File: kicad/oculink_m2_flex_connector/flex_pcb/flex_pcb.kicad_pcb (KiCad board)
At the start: 2 copper layers, 42 x 20 mm, 3 parts, among them J1 Conn_02x01, J2 Conn_02x01

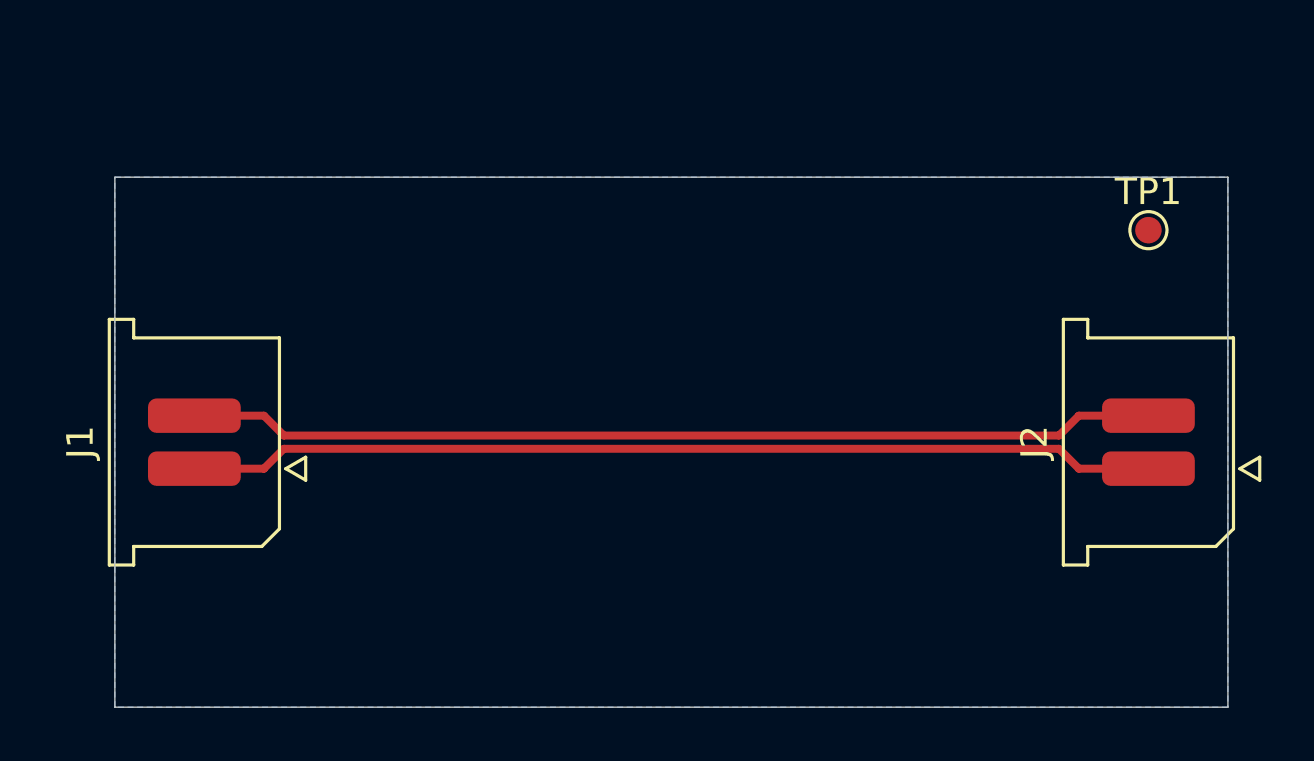
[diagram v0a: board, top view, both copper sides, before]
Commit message: Crude flex pcb layout
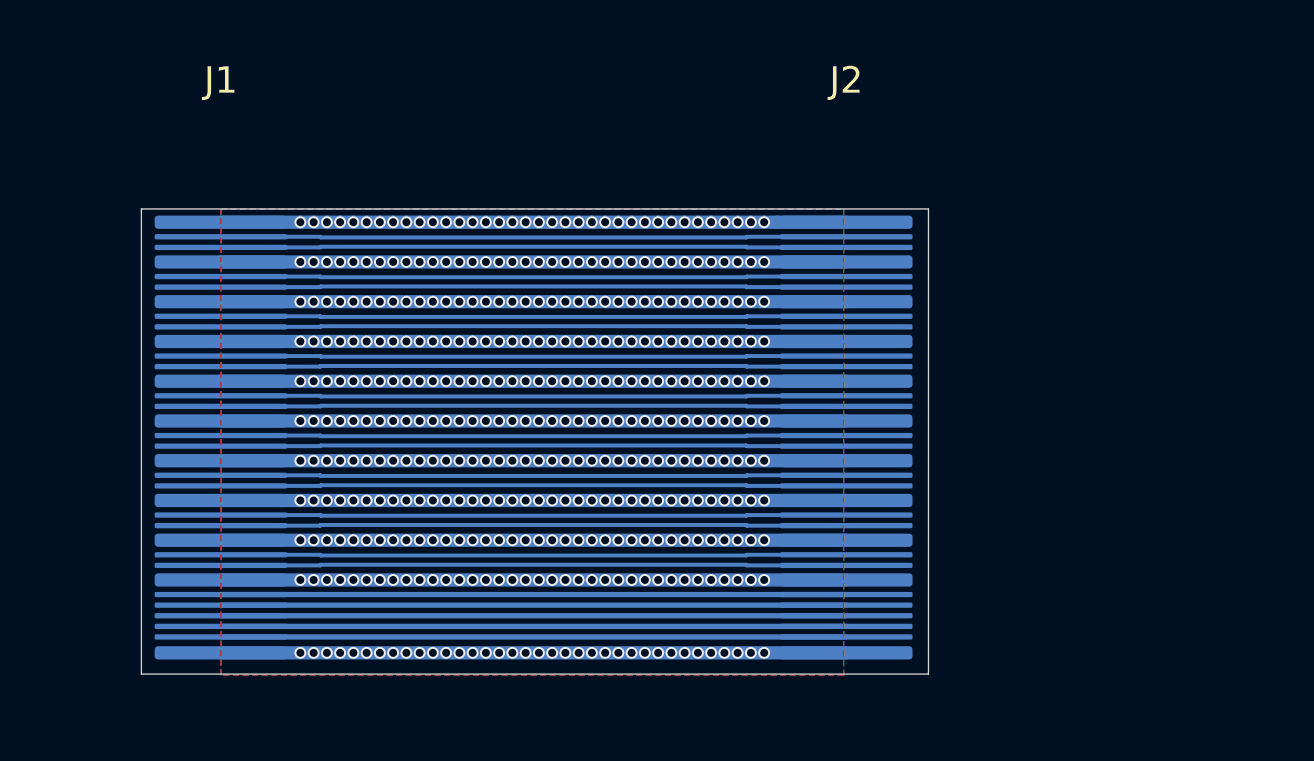
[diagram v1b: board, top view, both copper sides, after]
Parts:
- removed TP1: TestPoint, TestPoint:TestPoint_Pad_D1.0mm
- J1, J2: value Conn_02x01 -> Conn_01x38_Pin; footprint Connector_Samtec_MicroPower:Samtec_UMPS-02-XX.X-X-V-S_1x02_P2.0mm_Socket -> flex_connector:port_pcb
- moved J2 17.4 mm to (117.6, 66.8), turned to 0 degrees
- moved J1 13.2 mm to (94.0, 66.8), turned to 0 degrees
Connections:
- net D- renamed CLOCK+
- J1 pad 1: D+ -> GND
- J2 pad 1: D+ -> GND
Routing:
- net GND: track 0.00 -> 259.6 mm, vias 0 -> 396
- net D+: track 36.6 -> 0.00 mm
- net TX3-: track 0.00 -> 23.6 mm
- net TX3+: track 0.00 -> 23.6 mm
- net TX2-: track 0.00 -> 23.6 mm
- net TX2+: track 0.00 -> 23.6 mm
- net TX1-: track 0.00 -> 23.6 mm
- net TX1+: track 0.00 -> 23.6 mm
- net TX0-: track 0.00 -> 23.6 mm
- net TX0+: track 0.00 -> 23.6 mm
- net RX3-: track 0.00 -> 23.6 mm
- net RX3+: track 0.00 -> 23.6 mm
- net RX2-: track 0.00 -> 23.6 mm
- net RX2+: track 0.00 -> 23.6 mm
- net RX1-: track 0.00 -> 23.6 mm
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- added copper zone on F.Cu, net GND
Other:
- board size 42 x 20 mm -> 29.7 x 17.5 mm

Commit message: Test design for consistent hatched ground plane
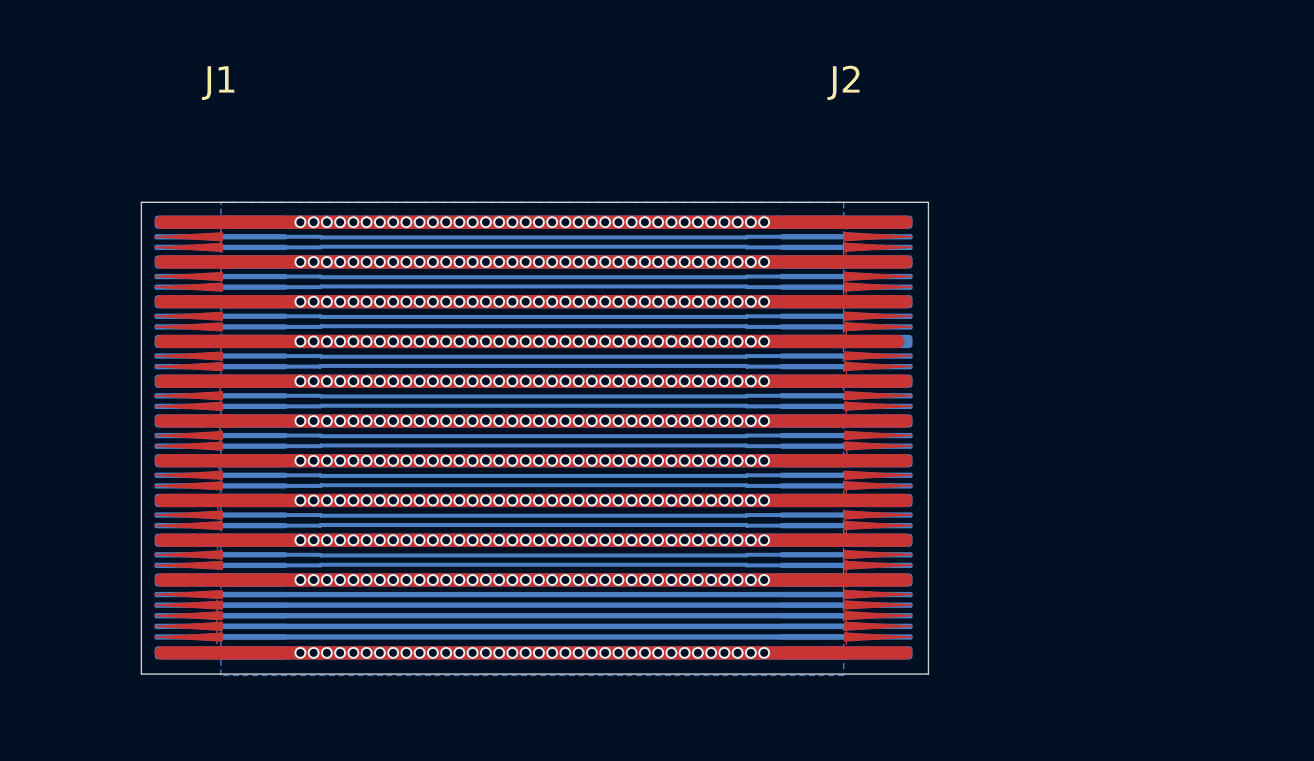
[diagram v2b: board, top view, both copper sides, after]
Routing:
- net GND: track 259.6 -> 569.0 mm
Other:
- board size 29.7 x 17.5 mm -> 29.7 x 17.8 mm
